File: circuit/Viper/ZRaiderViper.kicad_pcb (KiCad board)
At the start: 2 copper layers, 168 x 102 mm, 33 parts, among them J1 DE9_Socket, J2 DE9_Socket, SW1 TRIGGER_1, SW10 DOWN_2, SW11 LEFT_2, SW2 TRIGGER_2, SW3 Calibrate, SW4 UP_1, SW5 DOWN_1, SW6 LEFT_1, SW7 RIGHT_1, SW8 RIGHT_2, SW9 UP_2

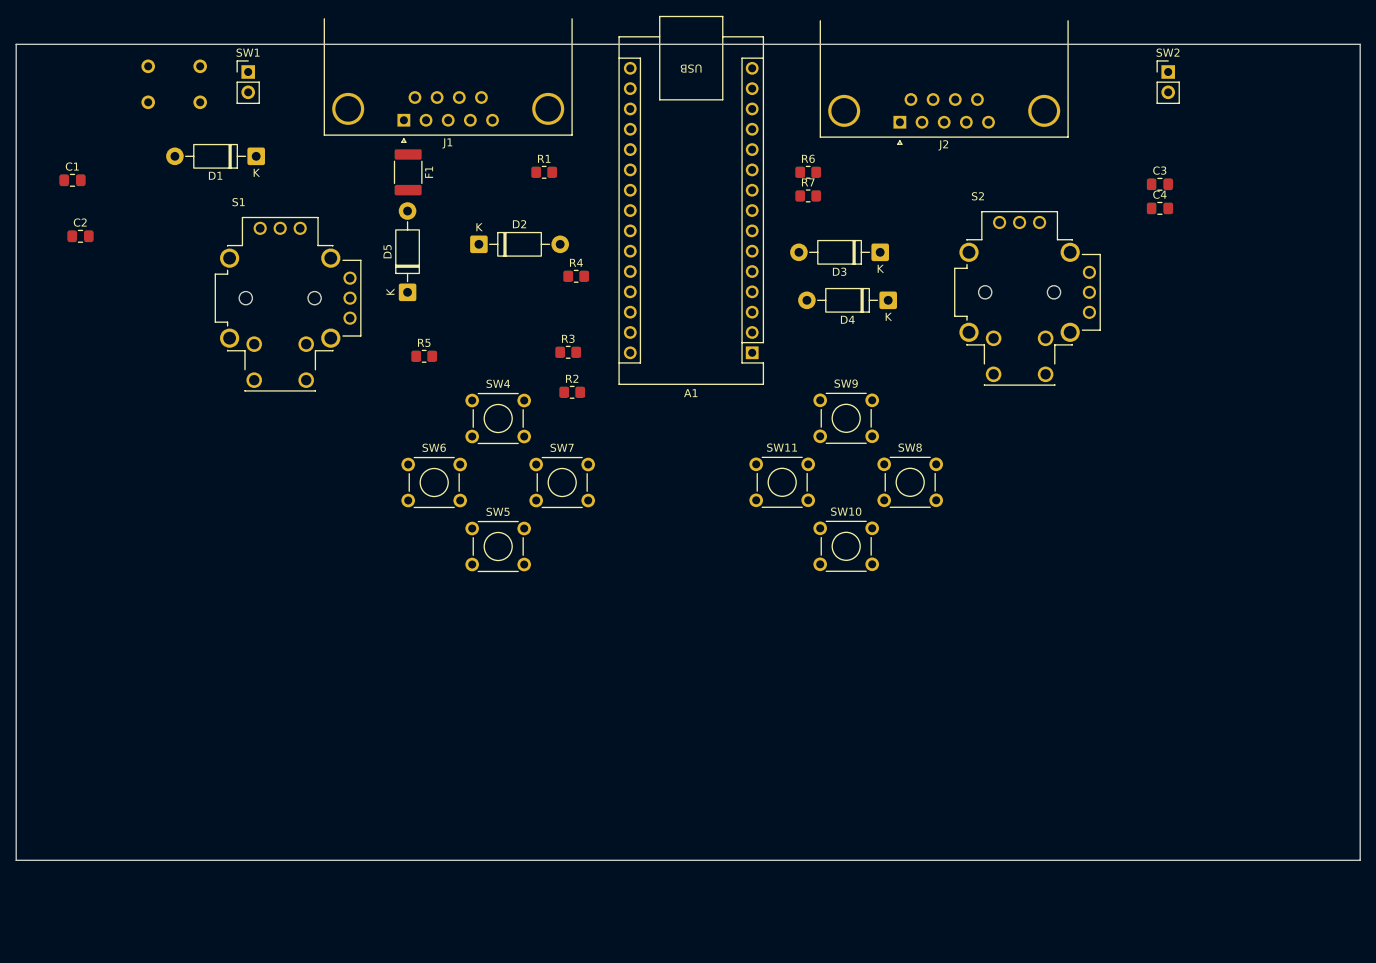
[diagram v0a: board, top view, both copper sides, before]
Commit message: working on viper PCB layout
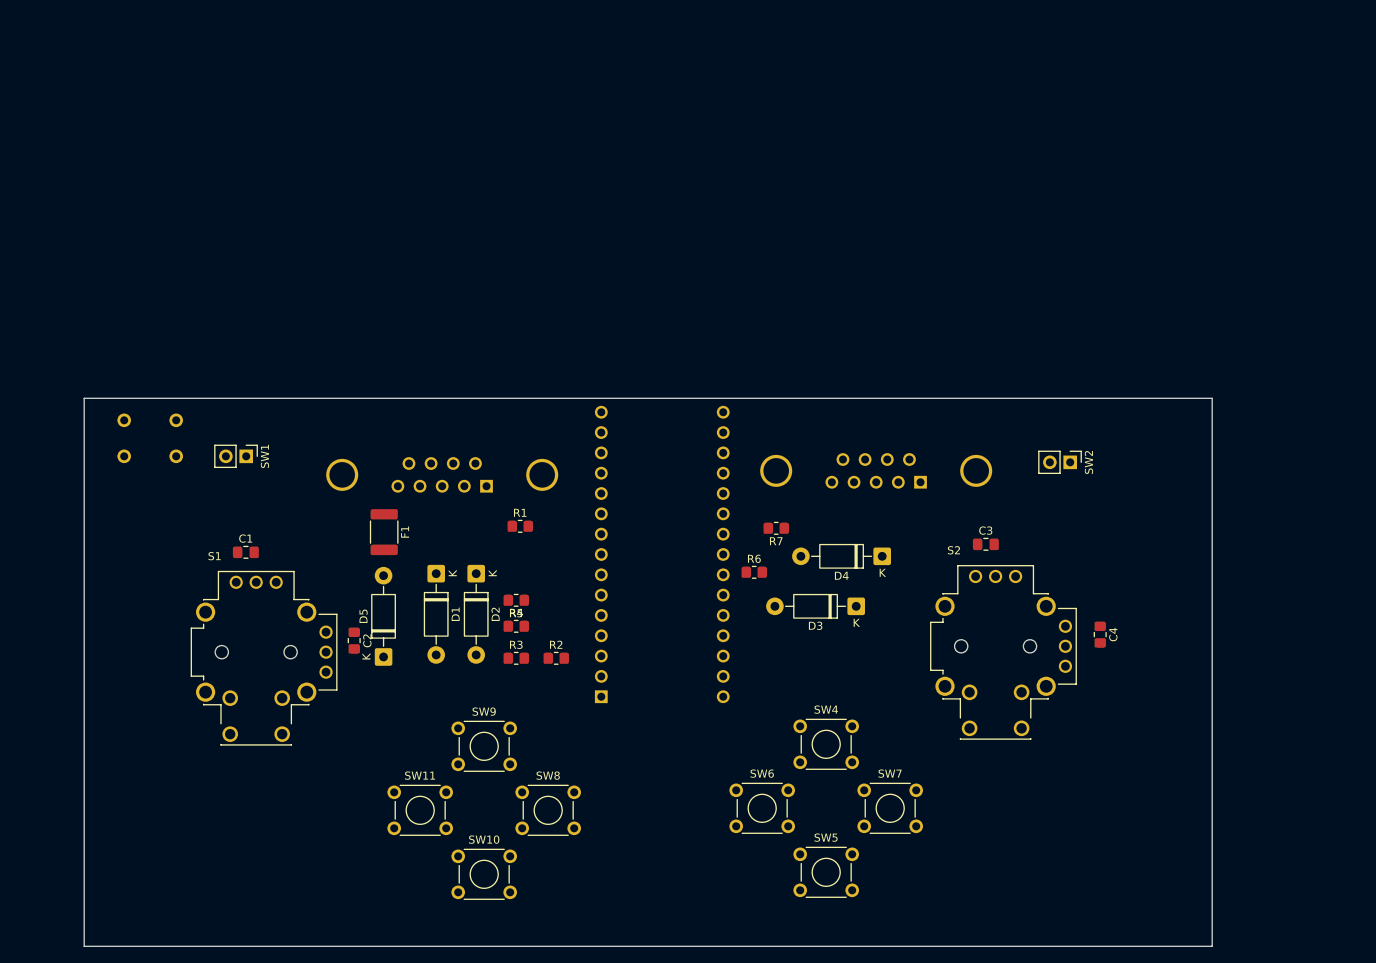
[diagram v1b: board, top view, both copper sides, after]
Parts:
- A1, J1, J2: moved to B.Cu
- moved SW10 61.1 mm to (121.2, 128.5)
- moved SW11 61.1 mm to (113.2, 120.5)
- moved SW8 61.1 mm to (129.2, 120.5)
- moved SW9 61.1 mm to (121.2, 112.5)
- moved C2 61.0 mm to (108.2, 101.5), turned to -90 degrees
- moved SW4 57.8 mm to (164.0, 112.2)
- moved SW5 57.8 mm to (164.0, 128.2)
- moved SW6 57.8 mm to (156.0, 120.2)
- moved SW7 57.8 mm to (172.0, 120.2)
- moved D1 56.8 mm to (118.5, 93.2), turned to -90 degrees
- moved C4 53.8 mm to (201.5, 100.8), turned to -90 degrees
- moved C1 51.3 mm to (94.7, 90.5)
- moved R6 50.5 mm to (158.2, 93.0)
- moved SW2 50.3 mm to (197.8, 79.2), turned to -90 degrees
- moved C3 50.0 mm to (187.2, 89.5)
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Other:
- board size 168 x 102 mm -> 141 x 68.5 mm
